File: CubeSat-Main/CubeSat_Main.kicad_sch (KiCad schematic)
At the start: 20 parts, among them J1 Conn_01x03_Pin, J2 Conn_01x08_Socket, U1 STM32F411CEU6 - BlackPill, U2 LORA E220-900T22D, U3 BNO055, U4 LM35-LP, U5 GPS_NEO6M

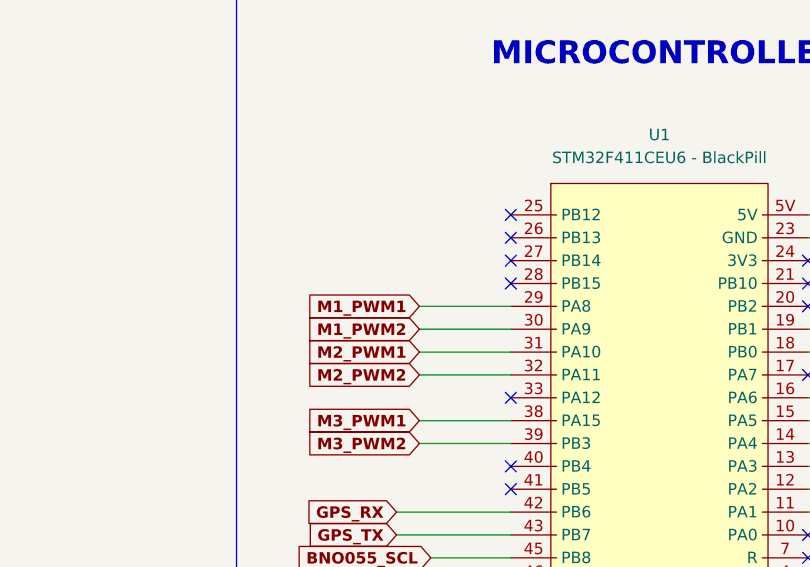
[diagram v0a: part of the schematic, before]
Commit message: small changes in layout
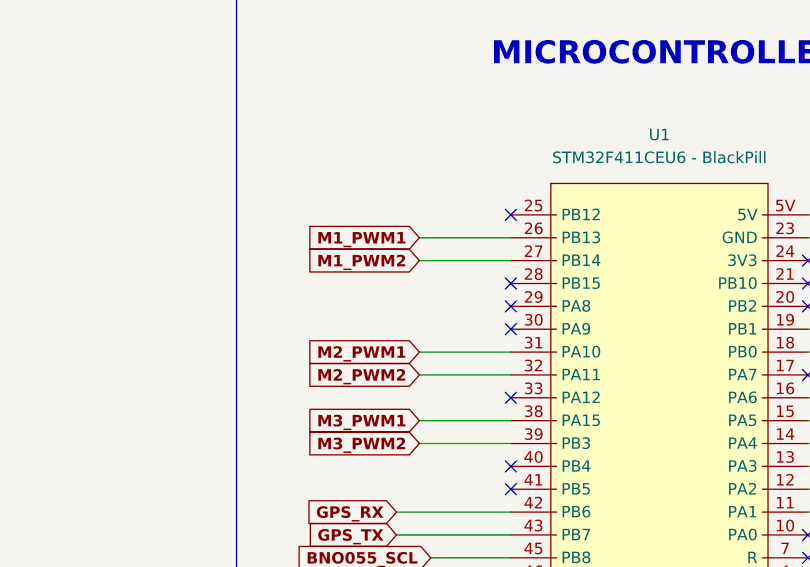
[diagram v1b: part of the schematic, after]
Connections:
- net M1_PWM1: now also U1.26 (PB13); no longer U1.29 (PA8)
- net M1_PWM2: now also U1.27 (PB14); no longer U1.30 (PA9)
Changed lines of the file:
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@@
+	)
+	(no_connect
+		(at 81.28 102.87)
 	)
 	(no_connect
@@
 	)
 	(no_connect
+		(at 81.28 105.41)
+	)
+	(no_connect
 		(at 257.81 144.78)
 	)
@@
 	)
 	(no_connect
-		(at 81.28 95.25)
-	)
-	(no_connect
-		(at 81.28 97.79)
-	)
-	(no_connect
 		(at 114.3 138.43)
 	)
@@
 	(wire
 		(pts
+			(xy 71.12 97.79) (xy 81.28 97.79)
+		)
+		(stroke
+			(width 0)
+			(type default)
+		)
+	)
+	(wire
+		(pts
 			(xy 71.12 107.95) (xy 81.28 107.95)
 		)
@@
 	(wire
 		(pts
-			(xy 71.12 105.41) (xy 81.28 105.41)
-		)
-		(stroke
-			(width 0)
-			(type default)
-		)
-	)
-	(wire
-		(pts
 			(xy 209.55 93.98) (xy 210.82 93.98)
 		)
@@
 	(wire
 		(pts
-			(xy 71.12 102.87) (xy 81.28 102.87)
-		)
-		(stroke
-			(width 0)
-			(type default)
-		)
-	)
-	(wire
-		(pts
 			(xy 68.58 125.73) (xy 81.28 125.73)
 		)
@@
 	(wire
 		(pts
+			(xy 71.12 95.25) (xy 81.28 95.25)
+		)
+		(stroke
+			(width 0)
+			(type default)
+		)
+	)
+	(wire
+		(pts
 			(xy 31.75 38.1) (xy 38.1 38.1)
 		)
@@
 	(global_label "M1_PWM1"
 		(shape input)
-		(at 71.12 102.87 180)
+		(at 71.12 95.25 180)
 		(fields_autoplaced yes)
 		(effects
@@
 		)
 		(property "Intersheetrefs" "${INTERSHEET_REFS}"
-			(at 58.648 102.87 0)
+			(at 58.648 95.25 0)
 			(effects
 				(font
@@
 	(global_label "M1_PWM2"
 		(shape input)
-		(at 71.12 105.41 180)
+		(at 71.12 97.79 180)
 		(fields_autoplaced yes)
 		(effects
@@
 		)
 		(property "Intersheetrefs" "${INTERSHEET_REFS}"
-			(at 58.648 105.41 0)
-			(effects
-				(font
+			(at 58.648 97.79 0)
+			(effects
+				(font
